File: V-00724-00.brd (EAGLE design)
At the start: 62 x 43.5 mm, 21 parts, among them IC1 MEGA8-AI, IC2 MAX481CSA, Q1 14.7456MHz, Q2 N-HEXFET_SOT323-IRLL014N

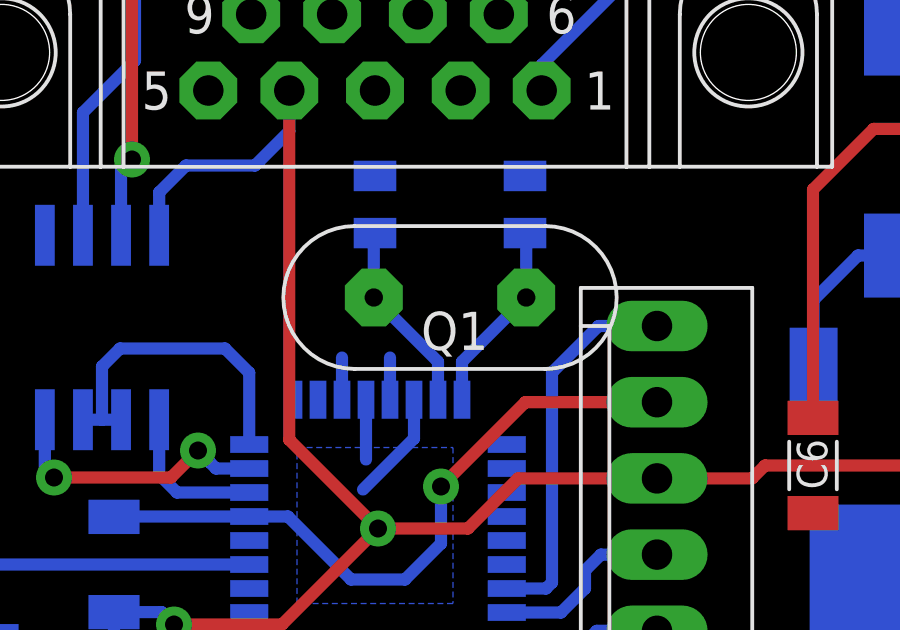
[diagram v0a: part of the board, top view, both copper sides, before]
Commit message: v1.1.0.2
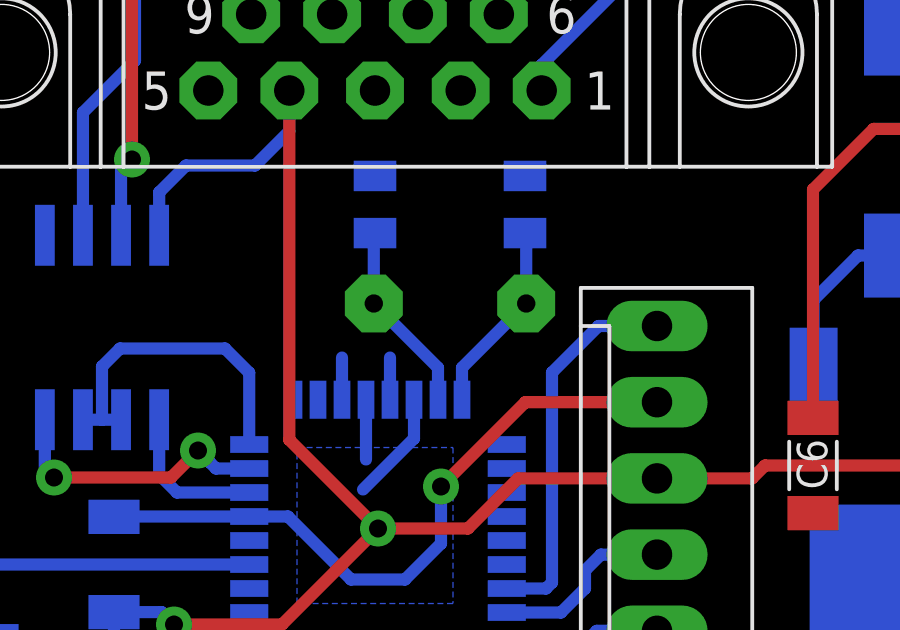
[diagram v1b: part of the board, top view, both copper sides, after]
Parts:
- moved Q1 0.20 mm to (31.9, 20.0), flipped to the bottom, turned to 0 degrees
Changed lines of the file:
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@@
 <layer number="14" name="Route14" color="1" fill="6" visible="no" active="yes"/>
 <layer number="15" name="Route15" color="4" fill="6" visible="no" active="yes"/>
-<layer number="16" name="Bottom" color="4" fill="1" visible="no" active="yes"/>
+<layer number="16" name="Bottom" color="4" fill="1" visible="yes" active="yes"/>
 <layer number="17" name="Pads" color="2" fill="1" visible="yes" active="yes"/>
 <layer number="18" name="Vias" color="2" fill="1" visible="yes" active="yes"/>
-<layer number="19" name="Unrouted" color="6" fill="1" visible="no" active="yes"/>
+<layer number="19" name="Unrouted" color="6" fill="1" visible="yes" active="yes"/>
 <layer number="20" name="Dimension" color="15" fill="1" visible="yes" active="yes"/>
-<layer number="21" name="tPlace" color="7" fill="1" visible="no" active="yes"/>
-<layer number="22" name="bPlace" color="7" fill="1" visible="no" active="yes"/>
-<layer number="23" name="tOrigins" color="15" fill="1" visible="no" active="yes"/>
-<layer number="24" name="bOrigins" color="15" fill="1" visible="no" active="yes"/>
-<layer number="25" name="tNames" color="7" fill="1" visible="no" active="yes"/>
-<layer number="26" name="bNames" color="7" fill="1" visible="no" active="yes"/>
-<layer number="27" name="tValues" color="7" fill="1" visible="no" active="yes"/>
-<layer number="28" name="bValues" color="7" fill="1" visible="no" active="yes"/>
+<layer number="21" name="tPlace" color="7" fill="1" visible="yes" active="yes"/>
+<layer number="22" name="bPlace" color="7" fill="1" visible="yes" active="yes"/>
+<layer number="23" name="tOrigins" color="15" fill="1" visible="yes" active="yes"/>
+<layer number="24" name="bOrigins" color="15" fill="1" visible="yes" active="yes"/>
+<layer number="25" name="tNames" color="7" fill="1" visible="yes" active="yes"/>
+<layer number="26" name="bNames" color="7" fill="1" visible="yes" active="yes"/>
+<layer number="27" name="tValues" color="7" fill="1" visible="yes" active="yes"/>
+<layer number="28" name="bValues" color="7" fill="1" visible="yes" active="yes"/>
 <layer number="29" name="tStop" color="7" fill="3" visible="no" active="yes"/>
 <layer number="30" name="bStop" color="7" fill="6" visible="no" active="yes"/>
@@
 <element name="R3" library="#PaJa_31" package="1206" value="10k" x="20.7" y="11.3" rot="MR270"/>
 <element name="C2" library="#PaJa_31" package="1206" value="10uF" x="39.5" y="1.7" rot="MR0"/>
-<element name="Q1" library="#PaJa_31" package="HC-49U" value="14.7456MHz" x="31.9" y="20.2" rot="R180"/>
+<element name="Q1" library="#PaJa_31" package="HC-49U" value="14.7456MHz" x="31.9" y="20" rot="MR0"/>
 <element name="C3" library="#PaJa_31" package="0805" value="27nF" x="29.4" y="23.3" rot="MR270"/>
 <element name="C4" library="#PaJa_31" package="0805" value="27nF" x="34.4" y="23.3" rot="MR270"/>
@@
 <contactref element="C3" pad="2"/>
 <contactref element="Q1" pad="2"/>
-<wire x1="31.5" y1="16.7926" x2="31.5" y2="18.06" width="0.4064" layer="16"/>
-<wire x1="31.5" y1="18.06" x2="29.36" y2="20.2" width="0.4064" layer="16"/>
-<wire x1="29.36" y1="20.2" x2="29.36" y2="22.3075" width="0.4064" layer="16"/>
+<wire x1="31.5" y1="16.7926" x2="31.5" y2="17.86" width="0.4064" layer="16"/>
+<wire x1="31.5" y1="17.86" x2="29.36" y2="20" width="0.4064" layer="16"/>
+<wire x1="29.36" y1="20" x2="29.36" y2="22.3075" width="0.4064" layer="16"/>
 <wire x1="29.36" y1="22.3075" x2="29.4" y2="22.3475" width="0.4064" layer="16"/>
 </signal>
@@
 <contactref element="Q1" pad="1"/>
 <contactref element="C4" pad="2"/>
-<wire x1="32.3" y1="16.7926" x2="32.3" y2="18.06" width="0.4064" layer="16"/>
-<wire x1="32.3" y1="18.06" x2="34.44" y2="20.2" width="0.4064" layer="16"/>
-<wire x1="34.44" y1="20.2" x2="34.44" y2="22.3075" width="0.4064" layer="16"/>
+<wire x1="32.3" y1="16.7926" x2="32.3" y2="17.86" width="0.4064" layer="16"/>
+<wire x1="32.3" y1="17.86" x2="34.44" y2="20" width="0.4064" layer="16"/>
+<wire x1="34.44" y1="20" x2="34.44" y2="22.3075" width="0.4064" layer="16"/>
 <wire x1="34.44" y1="22.3075" x2="34.4" y2="22.3475" width="0.4064" layer="16"/>
 </signal>
